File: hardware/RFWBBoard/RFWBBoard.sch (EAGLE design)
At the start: 95 parts, among them IC1 24LC025ST, J1 CON-71742-3003-BOT, M1 MOUNT-HOLE3.3, M2 MOUNT-HOLE3.3, M3 MOUNT-HOLE3.3, M4 MOUNT-HOLE3.3, M5 FIDUCIAL1X2, M6 FIDUCIAL1X2, M7 FIDUCIAL1X2, M8 FIDUCIAL1X2, U1 MAX2830IPC-7351, U2 LDB212G4010C-001, U3 LDB212G4010C-001, U4 AD8132MSOP8, U5 AD8132MSOP8, U6 AD8132MSOP8, U7 AD8132MSOP8, U8 LMV112, X1 SMA-SMD, X2 SMA-SMD, X3 FOX924B, X4 SMA-SMD, X5 SMA-SMD, X6 SMA-SMD, X7 SMA-SMD

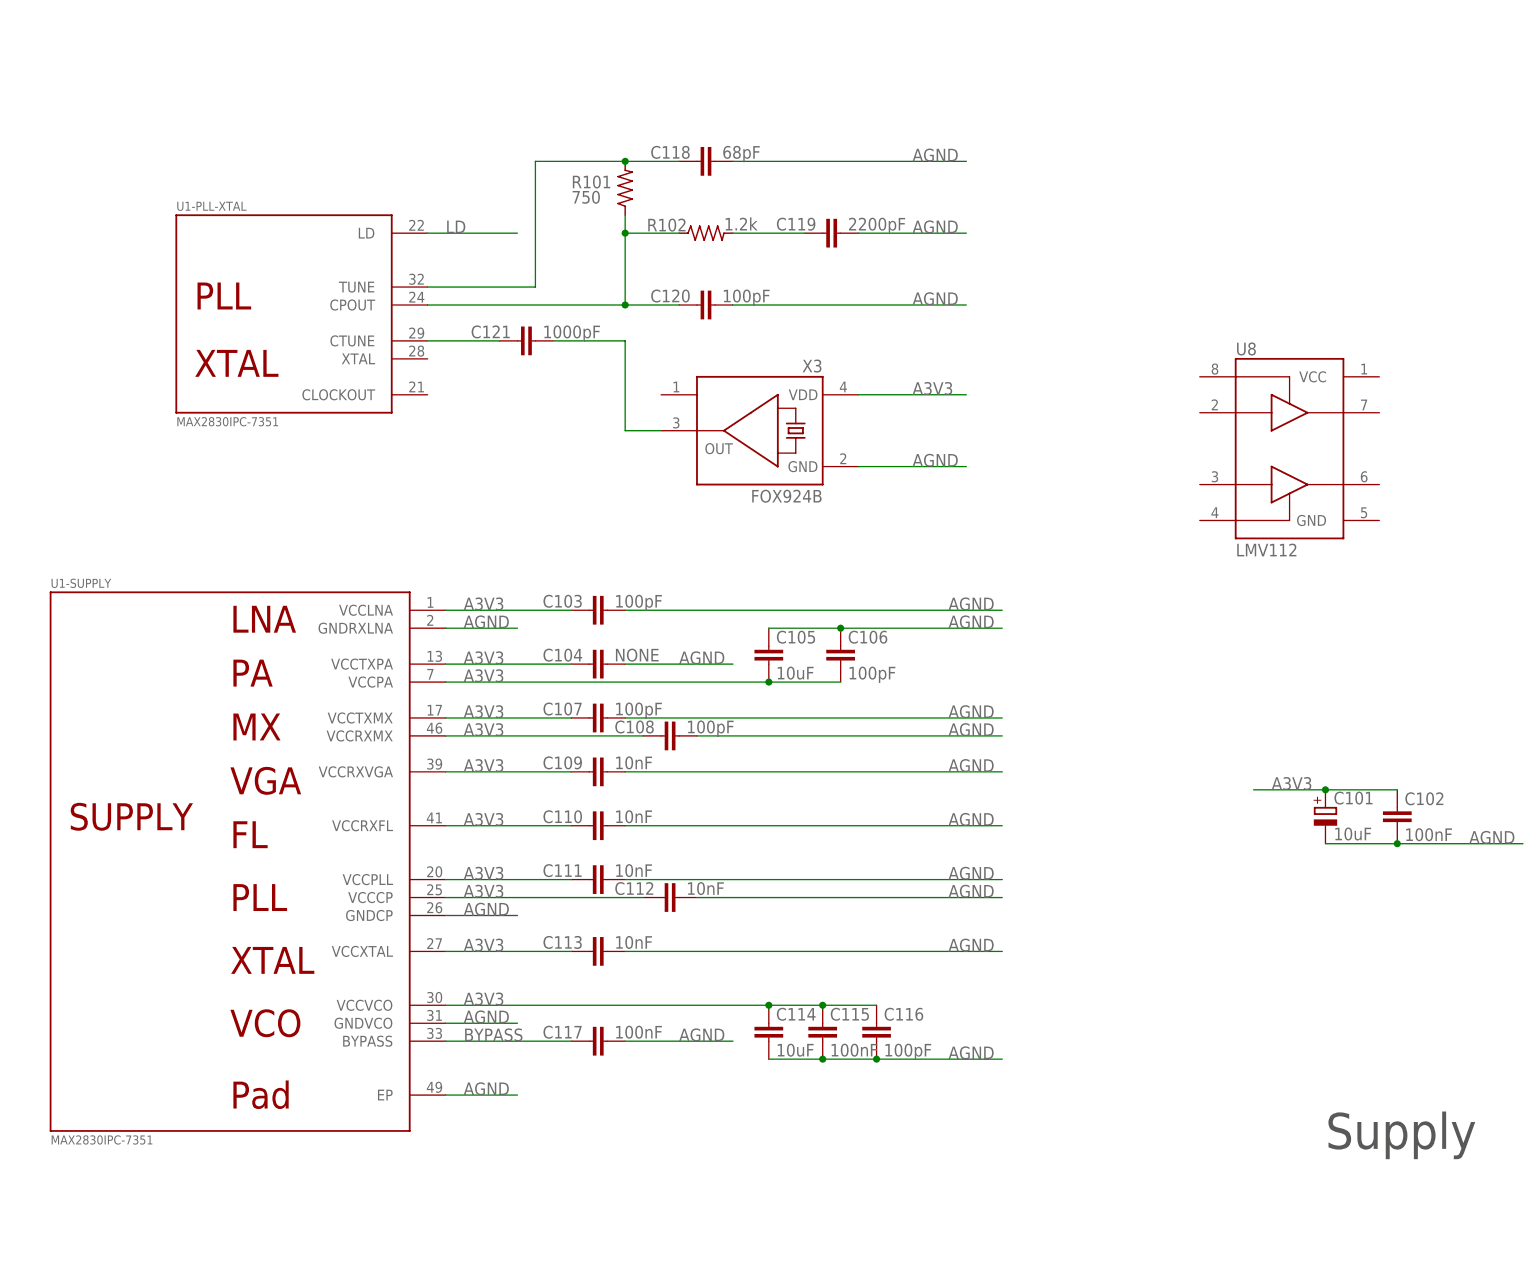
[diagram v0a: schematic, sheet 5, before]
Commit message: - Layout update
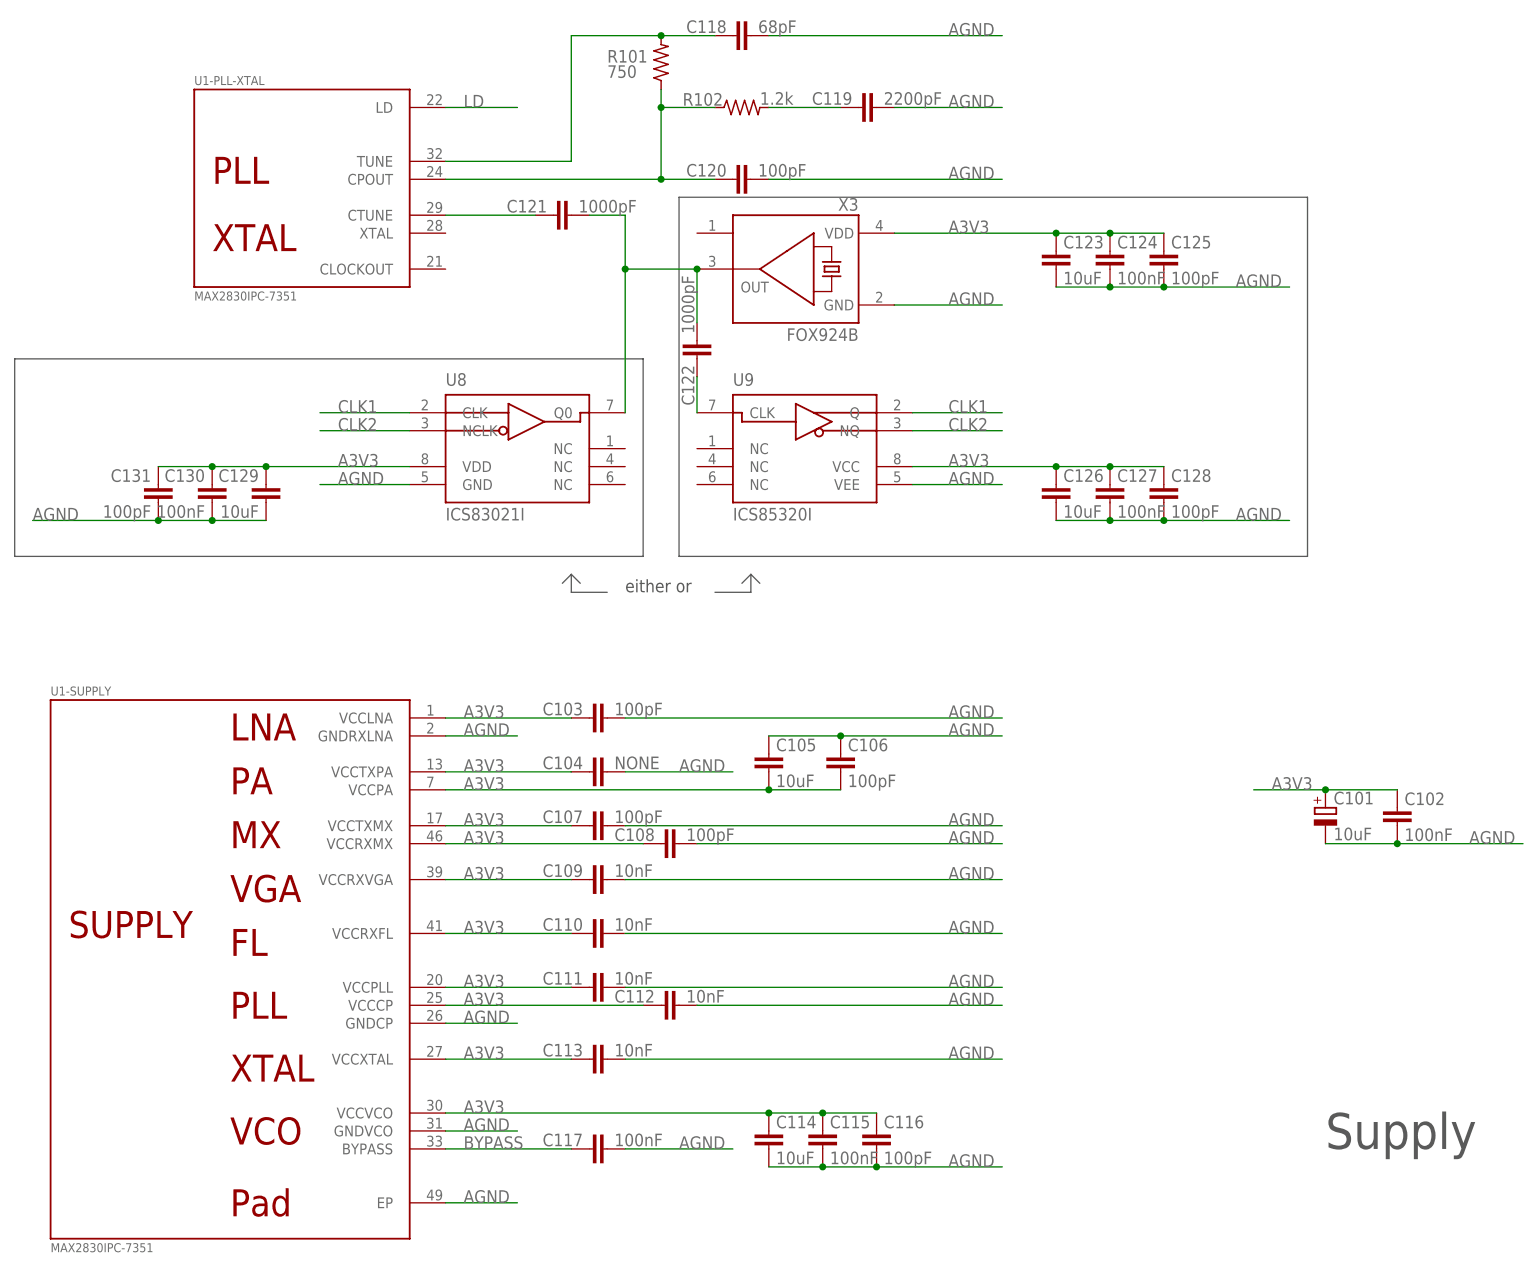
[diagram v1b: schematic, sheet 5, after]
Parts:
- added C122: 1000pF, RFWBBoard:C0402
- added C123, C126, C129: 10uF, RFWBBoard:C0805
- added C124, C127, C130: 100nF, RFWBBoard:C0402
- added C125, C128, C131: 100pF, RFWBBoard:C0402
- added U9: ICS85320I, RFWBBoard:ICS85320I
- U8: value LMV112 -> ICS83021I; device RFWBBoard:LMV112 -> RFWBBoard:ICS83021I
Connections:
- new net N$37: J1.11
- new net N$38: J1.13
- new net N$39: C122.1, U9.CLK
- new net N$40: J1.23
- new net N$41: J1.19
- new net N$42: J1.21
- net !SHDN: no longer J1.19
- net A3V3: now also C123.1, C124.1, C125.1, C126.1, C127.1, C128.1, C129.1, C130.1, C131.1, U8.VDD, U9.VCC
- net AGND: now also C123.2, C124.2, C125.2, C126.2, C127.2, C128.2, C129.2, C130.2, C131.2, U8.GND, U9.VEE
- net ANTSEL: no longer J1.13
- net CLK1: now also U8.CLK, U9.Q
- net CLK2: now also U8.NCLK, U9.NQ
- net LD: no longer J1.21
- net N$36: now also C122.2, U8.Q0
- net RXHP: no longer J1.11
- net RXTX: no longer J1.17
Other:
- note added: "either or"
- moved on the sheet: C103, C104, C105, C106, C107, C108, C109, C110, C111, C112, C113, C114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
